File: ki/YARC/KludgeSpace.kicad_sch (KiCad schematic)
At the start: 3 parts, among them J8 6-PIN FROM MCR, U100 74LS32, U101 74LS157

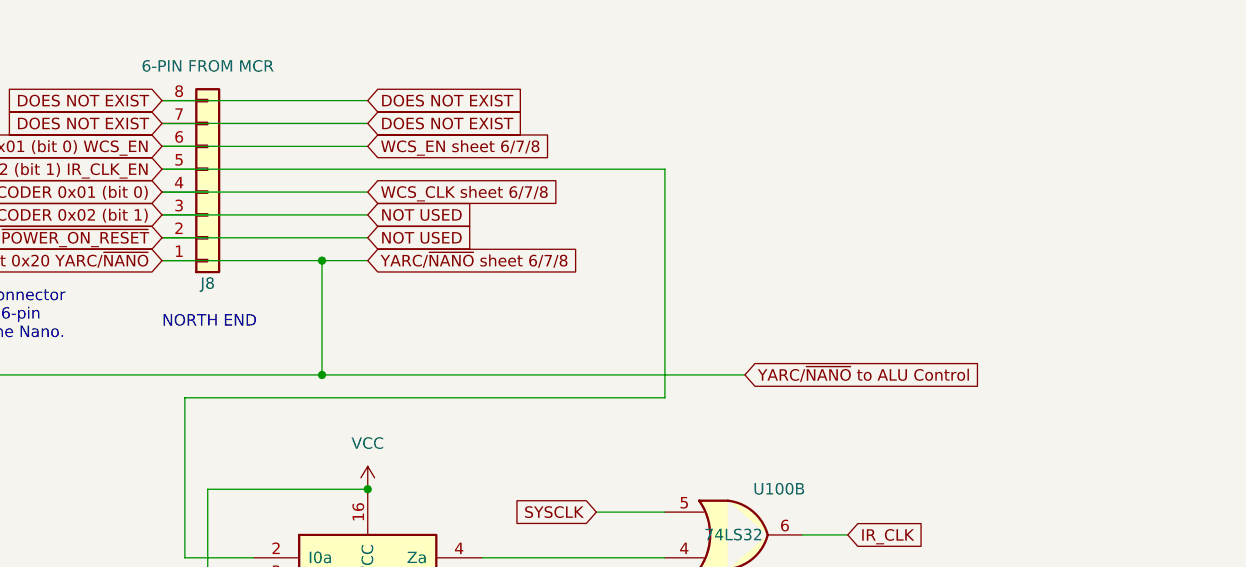
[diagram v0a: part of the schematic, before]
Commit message: Continuing corrections (only - no new functionality)
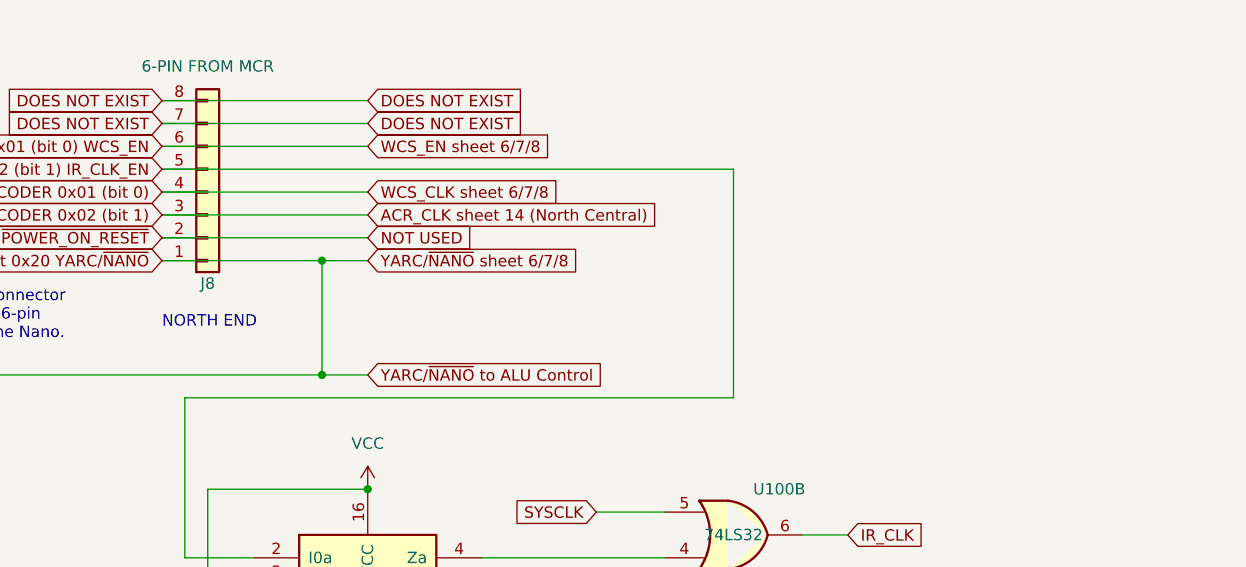
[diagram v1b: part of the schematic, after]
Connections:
- net ACR_CLK NANO DECODER 0x02 (bit 1): no longer J8.2 (Pin_2)
- new net NOT USED: J8.2 (Pin_2)
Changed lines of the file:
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@@
     (stroke (width 0) (type default) (color 0 0 0 0))
   )
-  (wire (pts (xy 111.76 43.18) (xy 55.88 43.18))
+  (wire (pts (xy 119.38 43.18) (xy 55.88 43.18))
     (stroke (width 0) (type default) (color 0 0 0 0))
   )
@@
     (stroke (width 0) (type default) (color 0 0 0 0))
   )
-  (wire (pts (xy 111.76 68.58) (xy 111.76 43.18))
+  (wire (pts (xy 119.38 68.58) (xy 119.38 43.18))
     (stroke (width 0) (type default) (color 0 0 0 0))
   )
@@
     (stroke (width 0) (type default) (color 0 0 0 0))
   )
-  (wire (pts (xy 73.66 66.04) (xy 120.65 66.04))
+  (wire (pts (xy 73.66 66.04) (xy 78.74 66.04))
     (stroke (width 0) (type default) (color 0 0 0 0))
   )
@@
     (stroke (width 0) (type default) (color 0 0 0 0))
   )
-  (wire (pts (xy 58.42 68.58) (xy 111.76 68.58))
+  (wire (pts (xy 58.42 68.58) (xy 119.38 68.58))
     (stroke (width 0) (type default) (color 0 0 0 0))
   )
@@
     )
   )
-  (global_label "YARC{slash}~{NANO} to ALU Control" (shape input) (at 120.65 66.04 0) (fields_autoplaced)
-    (effects (font (size 1.27 1.27)) (justify left))
-    (property "Intersheet References" "${INTERSHEET_REFS}" (id 0) (at 149.3098 65.9606 0)
+  (global_label "YARC{slash}~{NANO} to ALU Control" (shape input) (at 78.74 66.04 0) (fields_autoplaced)
+    (effects (font (size 1.27 1.27)) (justify left))
+    (property "Intersheet References" "${INTERSHEET_REFS}" (id 0) (at 107.3998 65.9606 0)
       (effects (font (size 1.27 1.27)) (justify left) hide)
     )
@@
     )
   )
-  (global_label "NOT USED" (shape input) (at 78.74 48.26 0) (fields_autoplaced)
-    (effects (font (size 1.27 1.27)) (justify left))
-    (property "Intersheet References" "${INTERSHEET_REFS}" (id 0) (at 90.7083 48.1806 0)
-      (effects (font (size 1.27 1.27)) (justify left) hide)
-    )
+  (global_label "ACR_CLK sheet 14 (North Central)" (shape input) (at 78.74 48.26 0) (fields_autoplaced)
+    (effects (font (size 1.27 1.27)) (justify left))
+    (property "Intersheet References" "${INTERSHEET_REFS}" (id 0) (at 114.3545 48.1806 0)
+      (effects (font (size 1.27 1.27)) (justify left) hide)
+    )
